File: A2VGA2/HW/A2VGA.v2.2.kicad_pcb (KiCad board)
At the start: 2 copper layers, 65.5 x 79.8 mm, 66 parts, among them U1 CPB

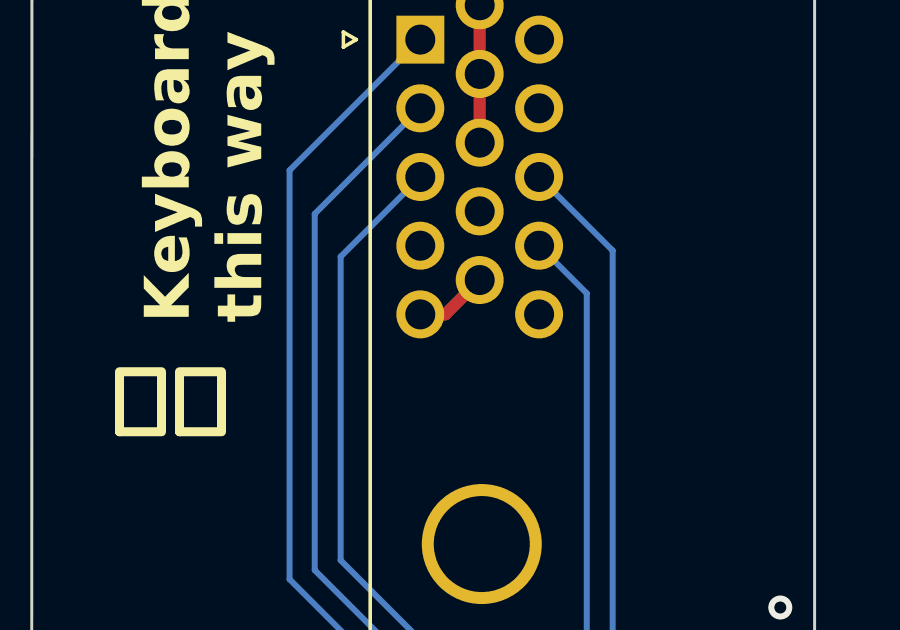
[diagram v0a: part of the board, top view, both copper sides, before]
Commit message: Add files via upload
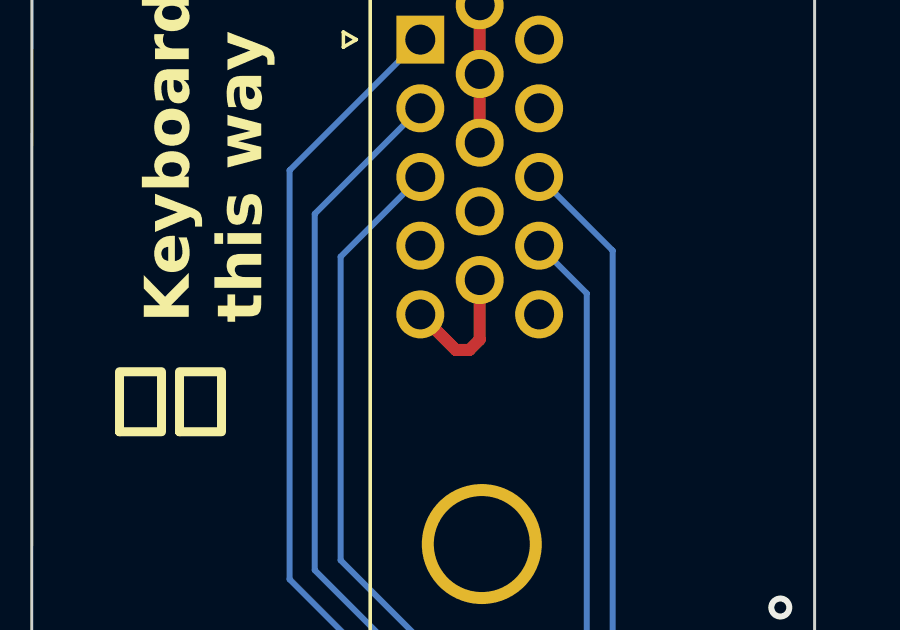
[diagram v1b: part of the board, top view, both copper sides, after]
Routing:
- net GND: track 12.0 -> 14.1 mm
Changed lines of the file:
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@@
 	)
 	(segment
-		(start 126.961869 79.3816)
-		(end 125.816869 80.5266)
+		(start 126.167069 81.7118)
+		(end 124.981869 80.5266)
+		(width 0.4)
+		(layer "F.Cu")
+		(net 1)
+	)
+	(segment
+		(start 126.961869 81.368931)
+		(end 126.619 81.7118)
 		(width 0.4)
 		(layer "F.Cu")
@@
 	)
 	(segment
-		(start 125.816869 80.5266)
-		(end 124.981869 80.5266)
+		(start 126.619 81.7118)
+		(end 126.167069 81.7118)
 		(width 0.4)
 		(layer "F.Cu")
+		(net 1)
+	)
+	(segment
+		(start 126.961869 79.3816)
+		(end 126.961869 81.368931)
+		(width 0.4)
+		(layer "F.Cu")
